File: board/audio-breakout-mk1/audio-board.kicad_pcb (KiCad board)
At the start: 2 copper layers, 24 x 21 mm, 2 parts, among them J1 Conn_01x06_Socket

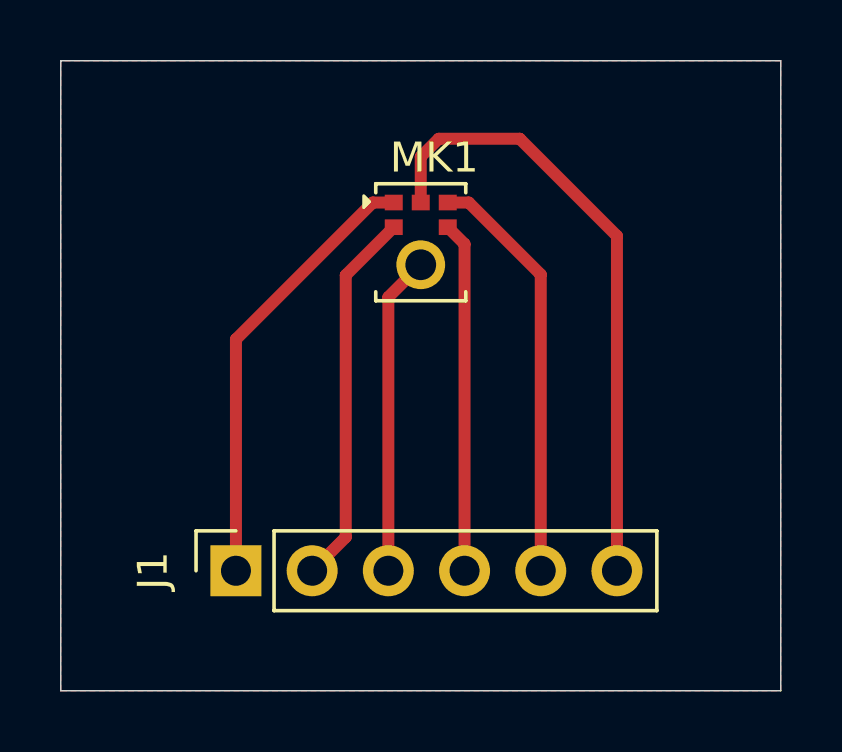
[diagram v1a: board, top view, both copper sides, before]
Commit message: archive
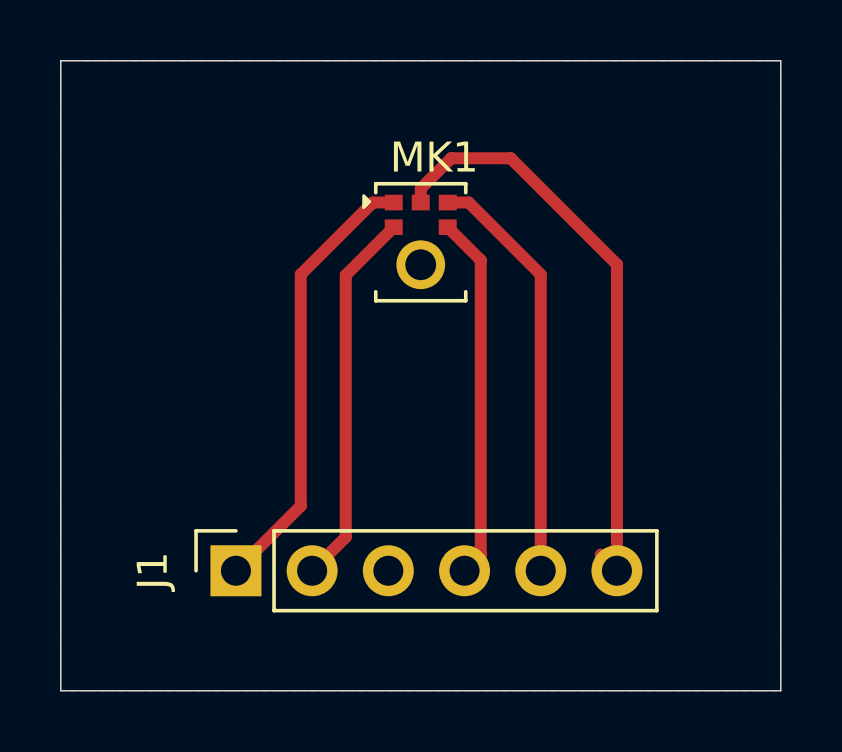
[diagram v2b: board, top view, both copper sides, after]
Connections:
- net Net-(J1-Pin_3) renamed GND
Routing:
- net GND: track 10.6 -> 0.00 mm
- net Net-(J1-Pin_6): track 20.8 -> 19.9 mm
- added copper zone on F.Cu, net GND
- removed copper zone on F.Cu, net (none)
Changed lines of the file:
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@@
 	(net 1 "Net-(J1-Pin_1)")
 	(net 2 "Net-(J1-Pin_6)")
-	(net 3 "Net-(J1-Pin_3)")
+	(net 3 "GND")
 	(net 4 "Net-(J1-Pin_4)")
 	(net 5 "Net-(J1-Pin_2)")
@@
 			(layers "*.Cu" "*.Mask")
 			(remove_unused_layers no)
-			(net 3 "Net-(J1-Pin_3)")
+			(net 3 "GND")
 			(pinfunction "Pin_3")
 			(pintype "passive")
@@
 			(layers "*.Cu" "*.Mask")
 			(remove_unused_layers no)
-			(net 3 "Net-(J1-Pin_3)")
+			(net 3 "GND")
 			(pinfunction "GND")
 			(pintype "power_in")
@@
 	)
 	(segment
+		(start 138 75.126)
+		(end 138 82.84)
+		(width 0.4)
+		(layer "F.Cu")
+		(net 1)
+	)
+	(segment
+		(start 138 82.84)
+		(end 135.84 85)
+		(width 0.4)
+		(layer "F.Cu")
+		(net 1)
+	)
+	(segment
+		(start 140.4 72.726)
+		(end 138 75.126)
+		(width 0.4)
+		(layer "F.Cu")
+		(net 1)
+	)
+	(segment
 		(start 141.1 72.726)
 		(end 140.4 72.726)
@@
 	)
 	(segment
-		(start 135.84 77.286)
-		(end 135.84 85)
-		(width 0.4)
-		(layer "F.Cu")
-		(net 1)
-	)
-	(segment
-		(start 140.4 72.726)
-		(end 135.84 77.286)
-		(width 0.4)
-		(layer "F.Cu")
-		(net 1)
-	)
-	(segment
-		(start 148.54 73.84)
+		(start 148.54 74.79)
+		(end 145 71.25)
+		(width 0.4)
+		(layer "F.Cu")
+		(net 2)
+	)
+	(segment
+		(start 148 84.46)
 		(end 148.54 85)
 		(width 0.4)
@@
 	)
 	(segment
-		(start 142 71.2)
-		(end 142.6 70.6)
+		(start 142 72.263)
+		(end 142 72.726)
 		(width 0.4)
 		(layer "F.Cu")
@@
 	)
 	(segment
-		(start 145.3 70.6)
-		(end 148.54 73.84)
+		(start 145 71.25)
+		(end 143.013 71.25)
 		(width 0.4)
 		(layer "F.Cu")
@@
 	)
 	(segment
-		(start 142.6 70.6)
-		(end 145.3 70.6)
+		(start 143.013 71.25)
+		(end 142 72.263)
 		(width 0.4)
 		(layer "F.Cu")
@@
 	)
 	(segment
-		(start 142 72.726)
-		(end 142 71.2)
+		(start 148.54 85)
+		(end 148.54 74.79)
 		(width 0.4)
 		(layer "F.Cu")
@@
 	)
 	(segment
-		(start 142 74.8)
-		(end 140.92 75.88)
-		(width 0.4)
-		(layer "F.Cu")
-		(net 3)
-	)
-	(segment
-		(start 140.92 75.88)
-		(end 140.92 85)
-		(width 0.4)
-		(layer "F.Cu")
-		(net 3)
+		(start 144 74.648)
+		(end 144 84.46)
+		(width 0.4)
+		(layer "F.Cu")
+		(net 4)
+	)
+	(segment
+		(start 144 84.46)
+		(end 143.46 85)
+		(width 0.4)
+		(layer "F.Cu")
+		(net 4)
 	)
 	(segment
 		(start 142.9 73.548)
-		(end 143.46 74.108)
-		(width 0.4)
-		(layer "F.Cu")
-		(net 4)
-	)
-	(segment
-		(start 143.46 74.108)
-		(end 143.46 85)
+		(end 144 74.648)
 		(width 0.4)
 		(layer "F.Cu")
@@
 	)
 	(segment
+		(start 143.6 72.726)
+		(end 146 75.126)
+		(width 0.4)
+		(layer "F.Cu")
+		(net 6)
+	)
+	(segment
 		(start 146 75.126)
 		(end 146 85)
@@
 		(net 6)
 	)
-	(segment
-		(start 143.6 72.726)
-		(end 146 75.126)
-		(width 0.4)
-		(layer "F.Cu")
-		(net 6)
-	)
 	(zone
-		(net 0)
-		(net_name "")
+		(net 3)
+		(net_name "GND")
 		(layer "F.Cu")
 		(hatch edge 0.5)
@@
 			(thermal_gap 0.5)
 			(thermal_bridge_width 0.5)
-			(island_removal_mode 1)
-			(island_area_min 10)
 		)
 		(polygon
